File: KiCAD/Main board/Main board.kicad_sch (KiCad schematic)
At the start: 29 parts, among them J1 Conn_01x03, J10 Conn_01x03, J11 Conn_01x03, J12 Conn_01x03, J13 Conn_01x02, J14 Conn_01x02, J15 Conn_01x06, J16 Conn_01x02, J17 Conn_01x02, J18 Conn_01x05, J2 Conn_01x03, J3 Conn_01x02, J4 Conn_01x02, J5 Conn_01x03, J6 Conn_01x02, J7 Conn_01x03, J8 Conn_01x02, J9 Conn_01x03

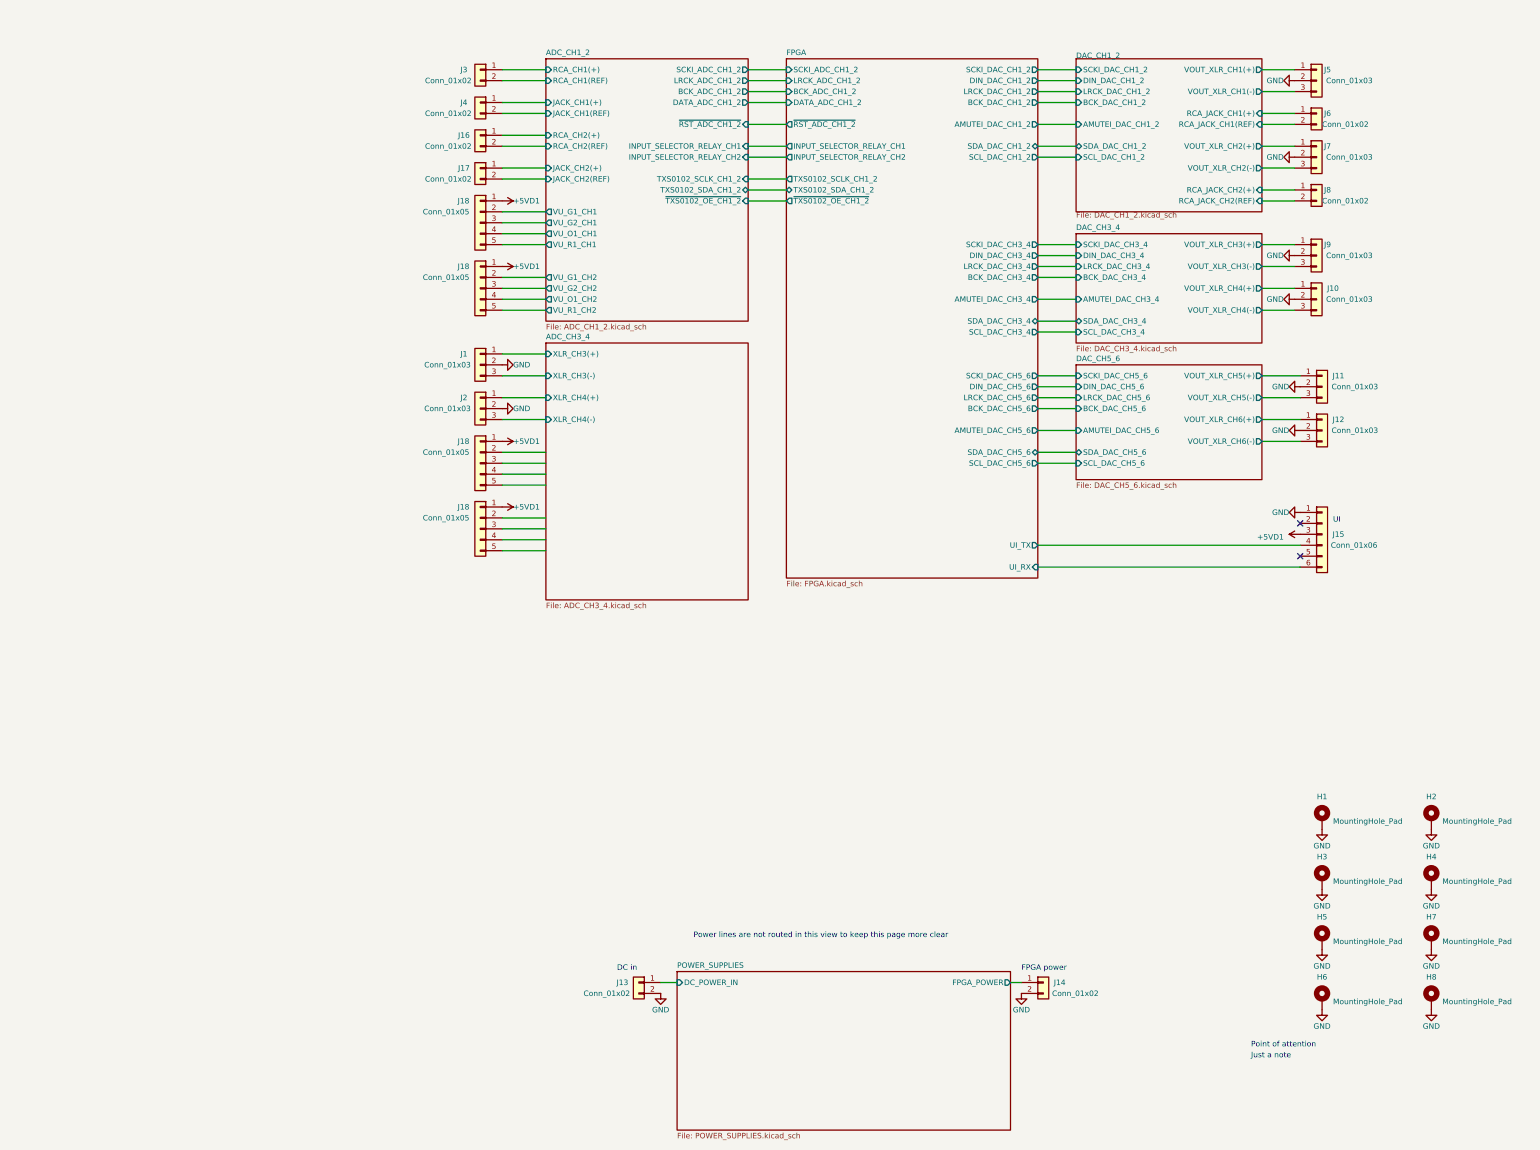
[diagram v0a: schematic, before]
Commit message: Worked on main board schematic
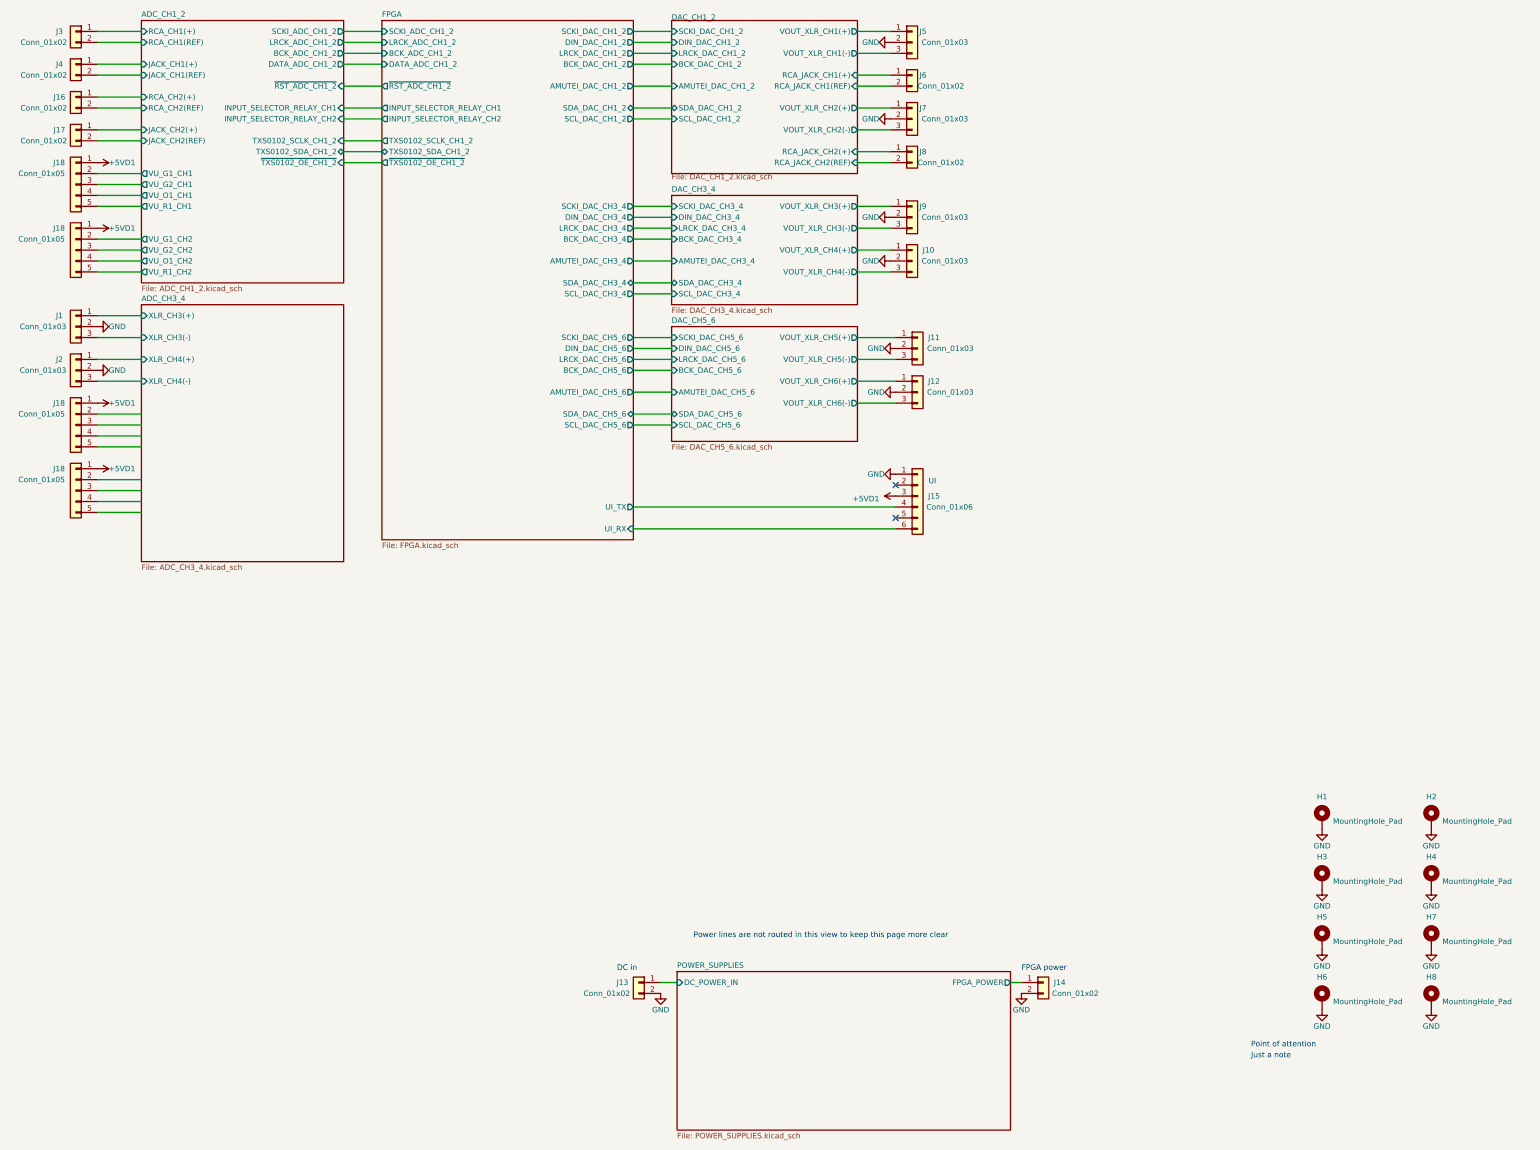
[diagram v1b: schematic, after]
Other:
- moved on the sheet: J1, J10, J11, J12, J15, J16, J17, J18, J2, J3, J4, J5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
